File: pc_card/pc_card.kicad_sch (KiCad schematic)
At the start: 44 parts, among them IC1 SV 3.3V, IC2 74LVC1G00, IC3 SV 4.5V, IC4 TPA152DR, J1 PCMCIA Connector, J2 Headphones Out, U1 Z8601720ASG, U2 25LCxxx, U3 YMF289B-S, U4 YAC516-E, Y1 4.19MHz, Y2 33.868MHz

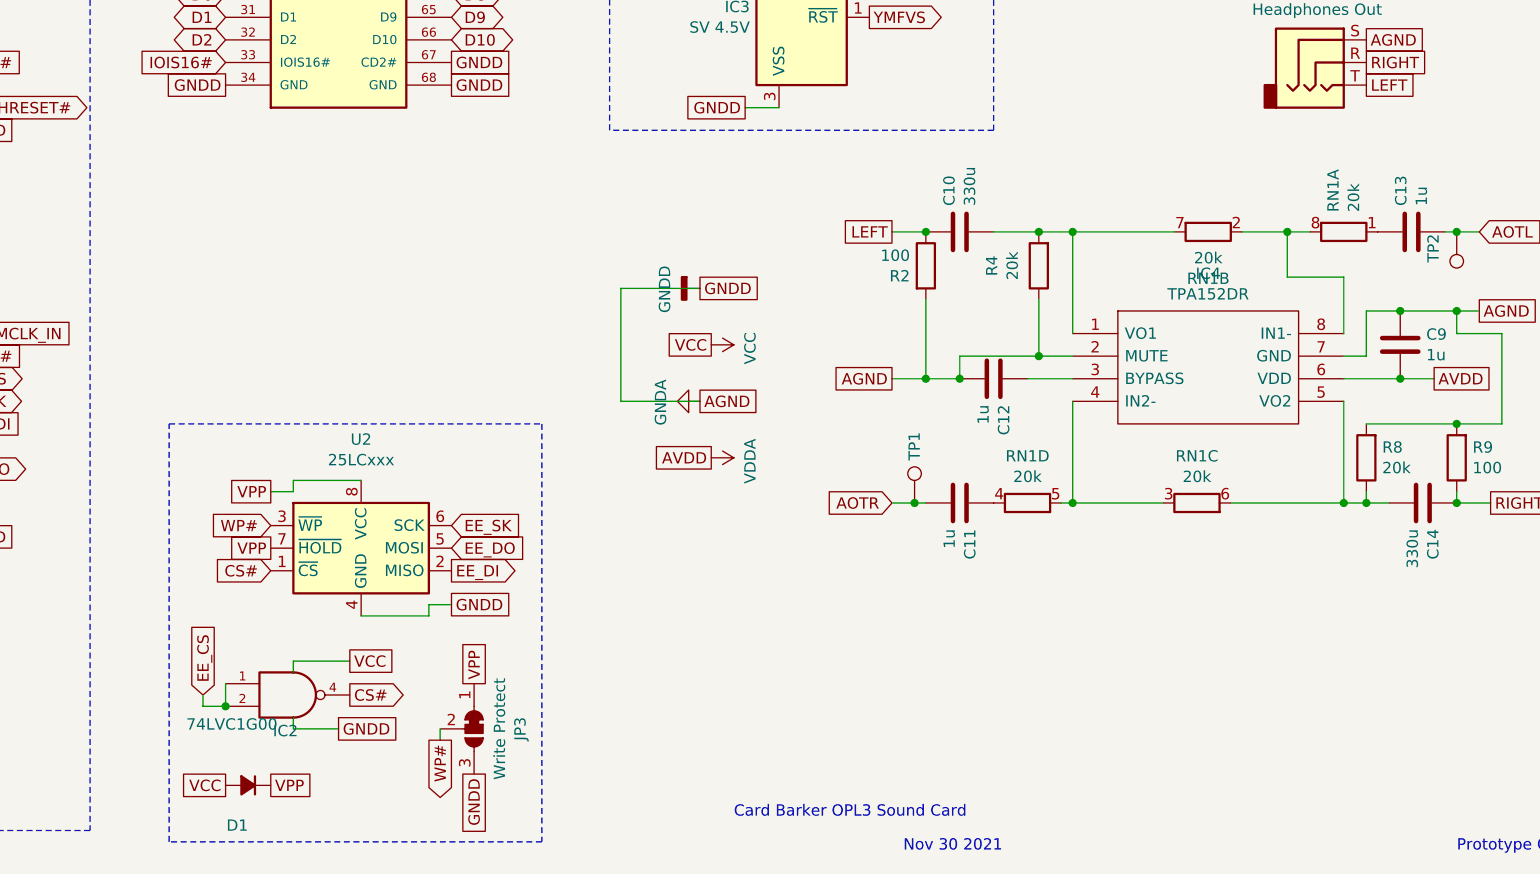
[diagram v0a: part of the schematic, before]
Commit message: fixes
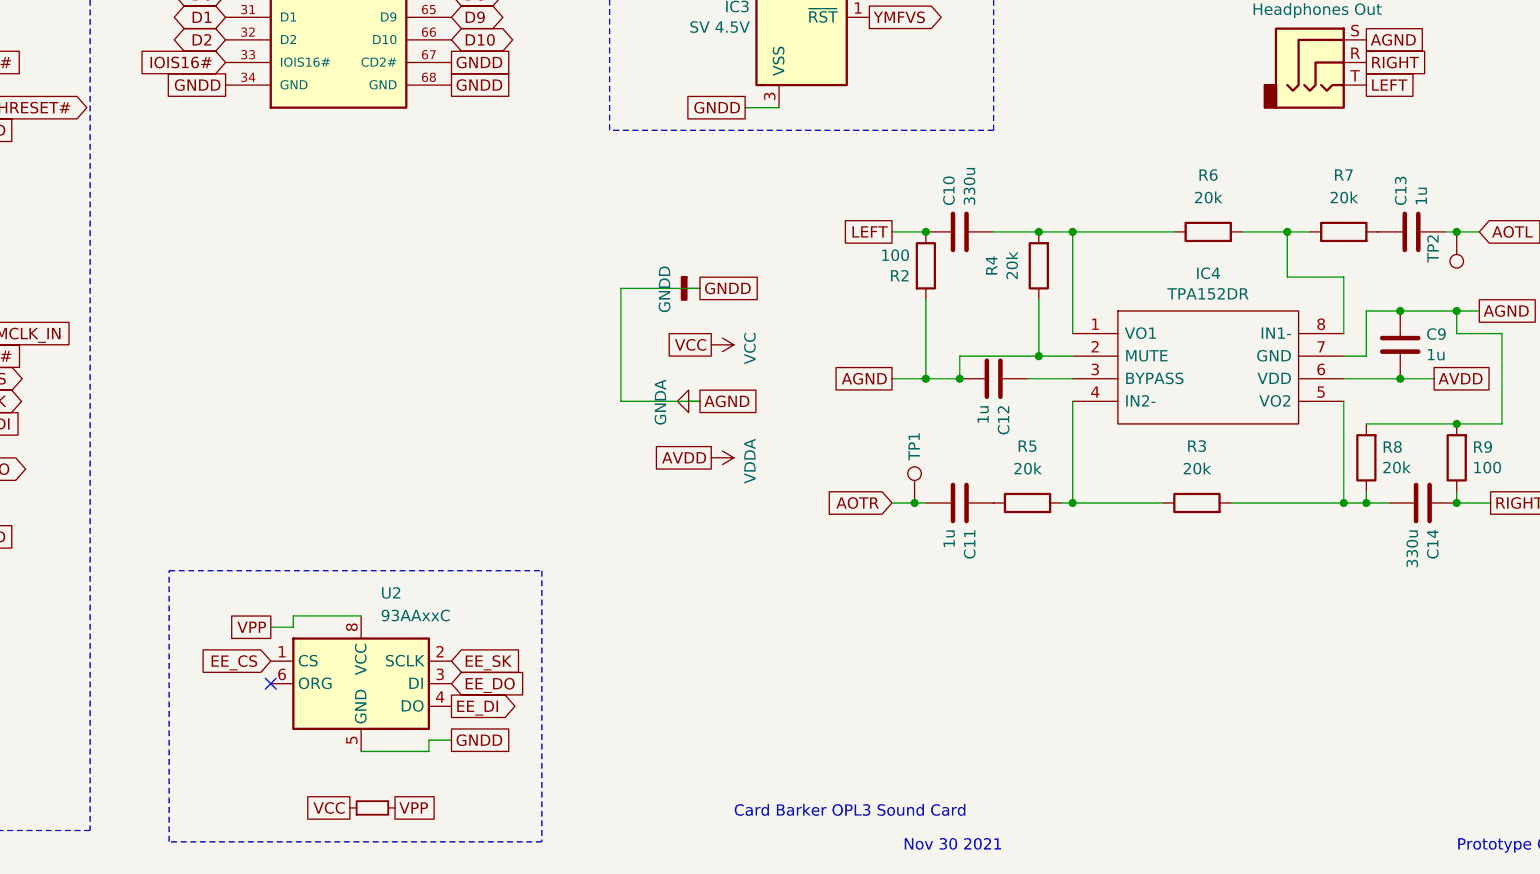
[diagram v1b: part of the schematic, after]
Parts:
- removed D1: D_Small_ALT, Diode_SMD:D_SOD-323_HandSoldering, symbol pc_card_sound_barker-rescue:D_Small_ALT-Device
- removed IC2: 74LVC1G00, Package_TO_SOT_SMD:SOT-23-5_HandSoldering, symbol pc_card_sound_barker-rescue:74LVC1G00-74xGxx
- removed JP3: Write Protect, Jumper:SolderJumper-3_P1.3mm_Bridged12_RoundedPad1.0x1.5mm_NumberLabels, symbol pc_card_sound_barker-rescue:SolderJumper_3_Bridged12-Jumper
- removed RN1: 20k, Resistor_SMD:R_Array_Convex_4x1206, symbol Device:R_Pack04_Split
- removed U2: 25LCxxx, Package_SO:SOIC-8_3.9x4.9mm_P1.27mm, symbol Memory_EEPROM:25LCxxx
- added R12: EEPROM, Resistor_SMD:R_0603_1608Metric_Pad0.98x0.95mm_HandSolder, symbol Device:R_Small
- added R3, R5, R6, R7: 20k, Resistor_SMD:R_0805_2012Metric_Pad1.20x1.40mm_HandSolder, symbol Device:R
- added U2: 93AAxxC, Package_SO:SOIC-8_3.9x4.9mm_P1.27mm, symbol Memory_EEPROM:93AAxxC
- IC4: footprint SOIC127P600X175-8N -> Package_SO:SOIC-8_3.9x4.9mm_P1.27mm
- U1: footprint QFP50P1600X1600X160-100N -> Package_QFP:LQFP-100_14x14mm_P0.5mm
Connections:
- net EE_CS: now also U2.1 (CS)
- net EE_DI: now also U2.4 (DO)
- net EE_DO: now also U2.3 (DI)
- net EE_SK: now also U2.2 (SCLK)
- net VCC: now also R12.1
- net VPP: now also R12.2, U2.8 (VCC)
- net at C13.1: now also R7.2
- net at IC4.8 (IN1-): now also R6.2, R7.1
- net at C10.2, IC4.1 (VO1), R4.2: now also R6.1
- net at IC4.4 (IN2-): now also R3.1, R5.2
- net at C14.2, IC4.5 (VO2), R8.1: now also R3.2
- net at C11.1: now also R5.1
- net GND renamed GNDA
- net GNDA: now also U2.5 (GND)
- no-connect marks 44 -> 45
